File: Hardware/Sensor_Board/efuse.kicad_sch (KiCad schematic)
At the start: 11 parts, among them U101 TPS25942ARVCR

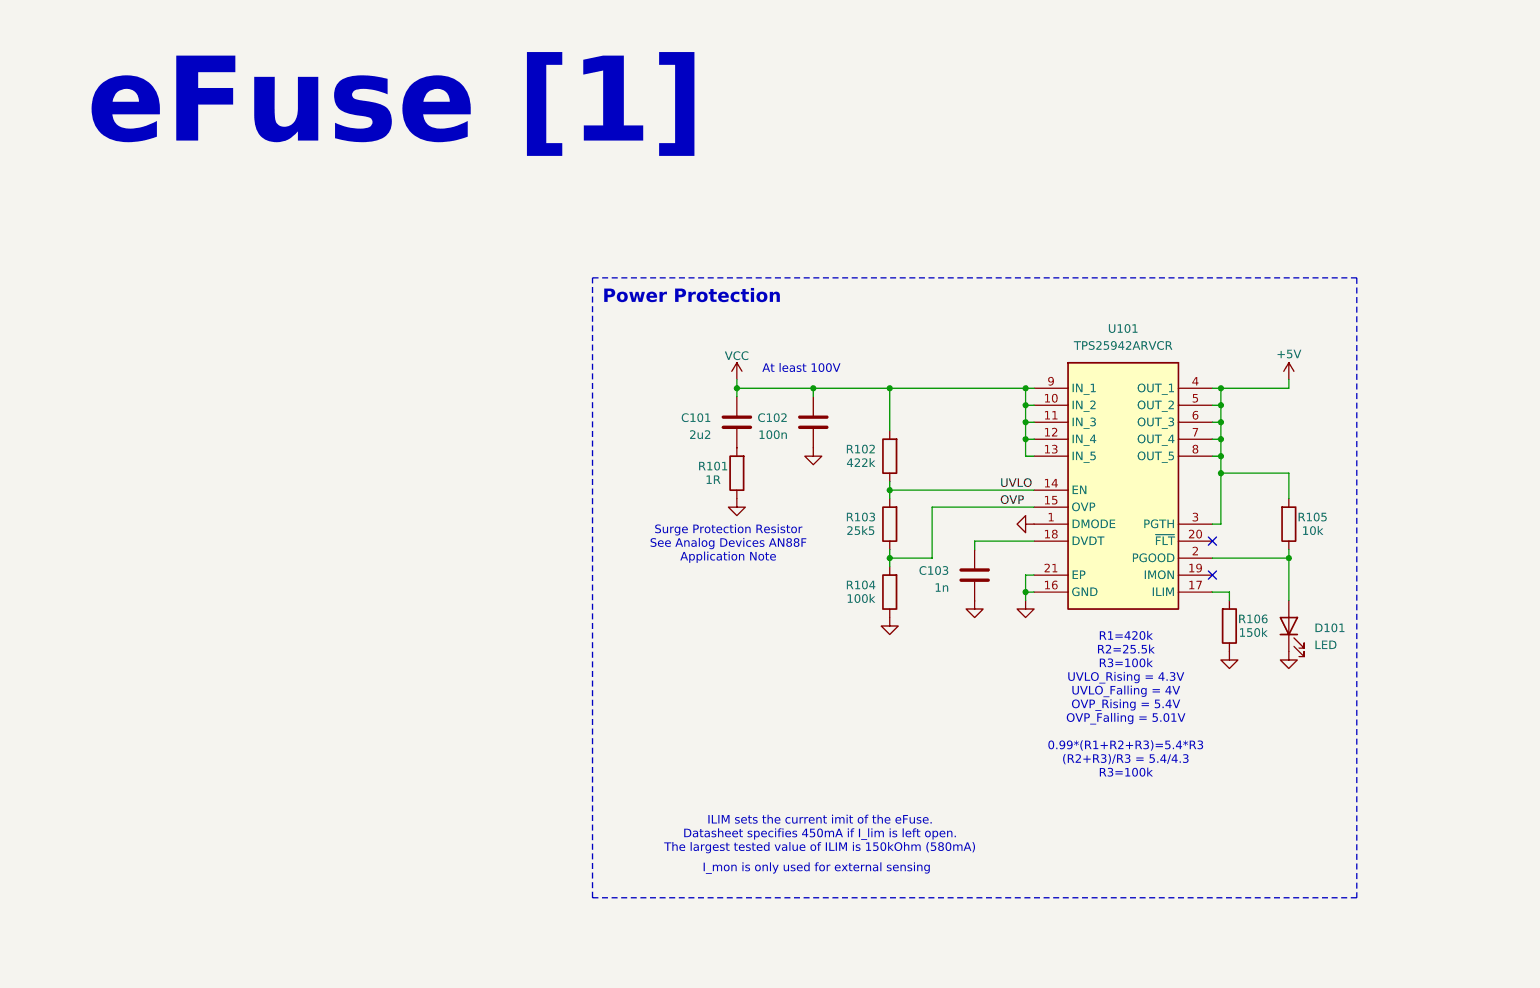
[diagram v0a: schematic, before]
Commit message: Finished design of both programmer and sensor board PCBs
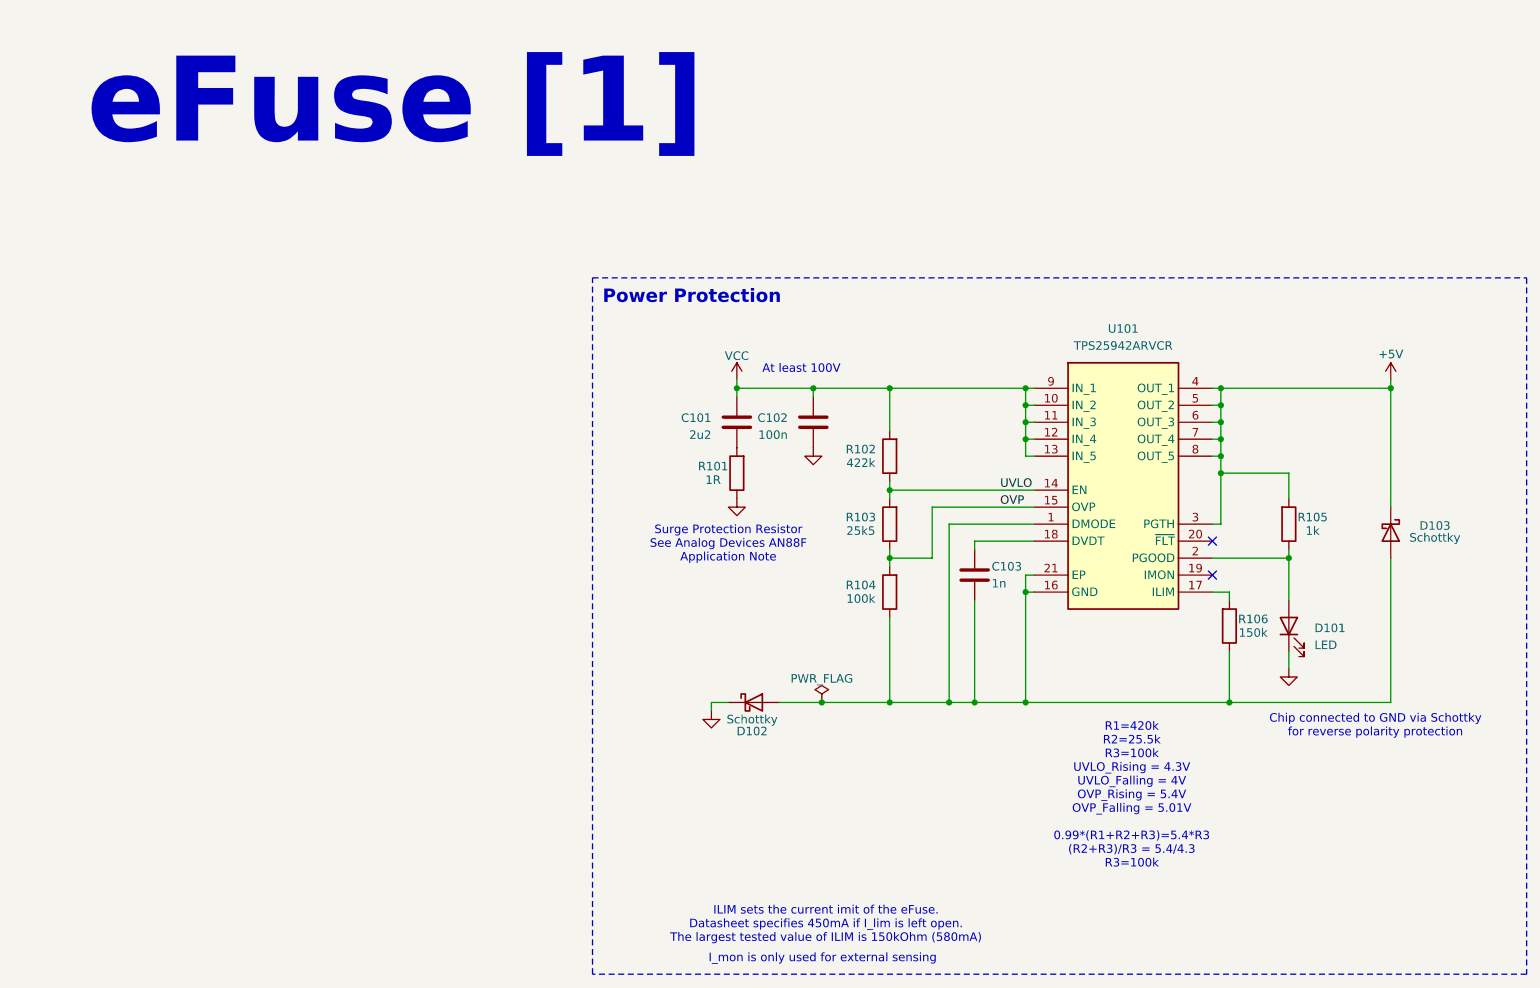
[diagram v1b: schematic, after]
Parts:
- added D102, D103: Schottky, Diode_SMD:D_0402_1005Metric, symbol Device:D_Schottky
- R105: value 10k -> 1k
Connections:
- net +5V: now also D103.1 (K)
- net GND: now also D102.1 (K); no longer C103.2, R104.1, R106.1, U101.1 (DMODE), U101.16 (GND), U101.21 (EP)
- new net: C103.2, D102.2 (A), D103.2 (A), R104.1, R106.1, U101.1 (DMODE), U101.16 (GND), U101.21 (EP)
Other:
- note added: "Chip connected to GND via Schottky for reverse polarity protection"
